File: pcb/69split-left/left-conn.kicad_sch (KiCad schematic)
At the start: 1 part, among them J1 USB_C_Receptacle

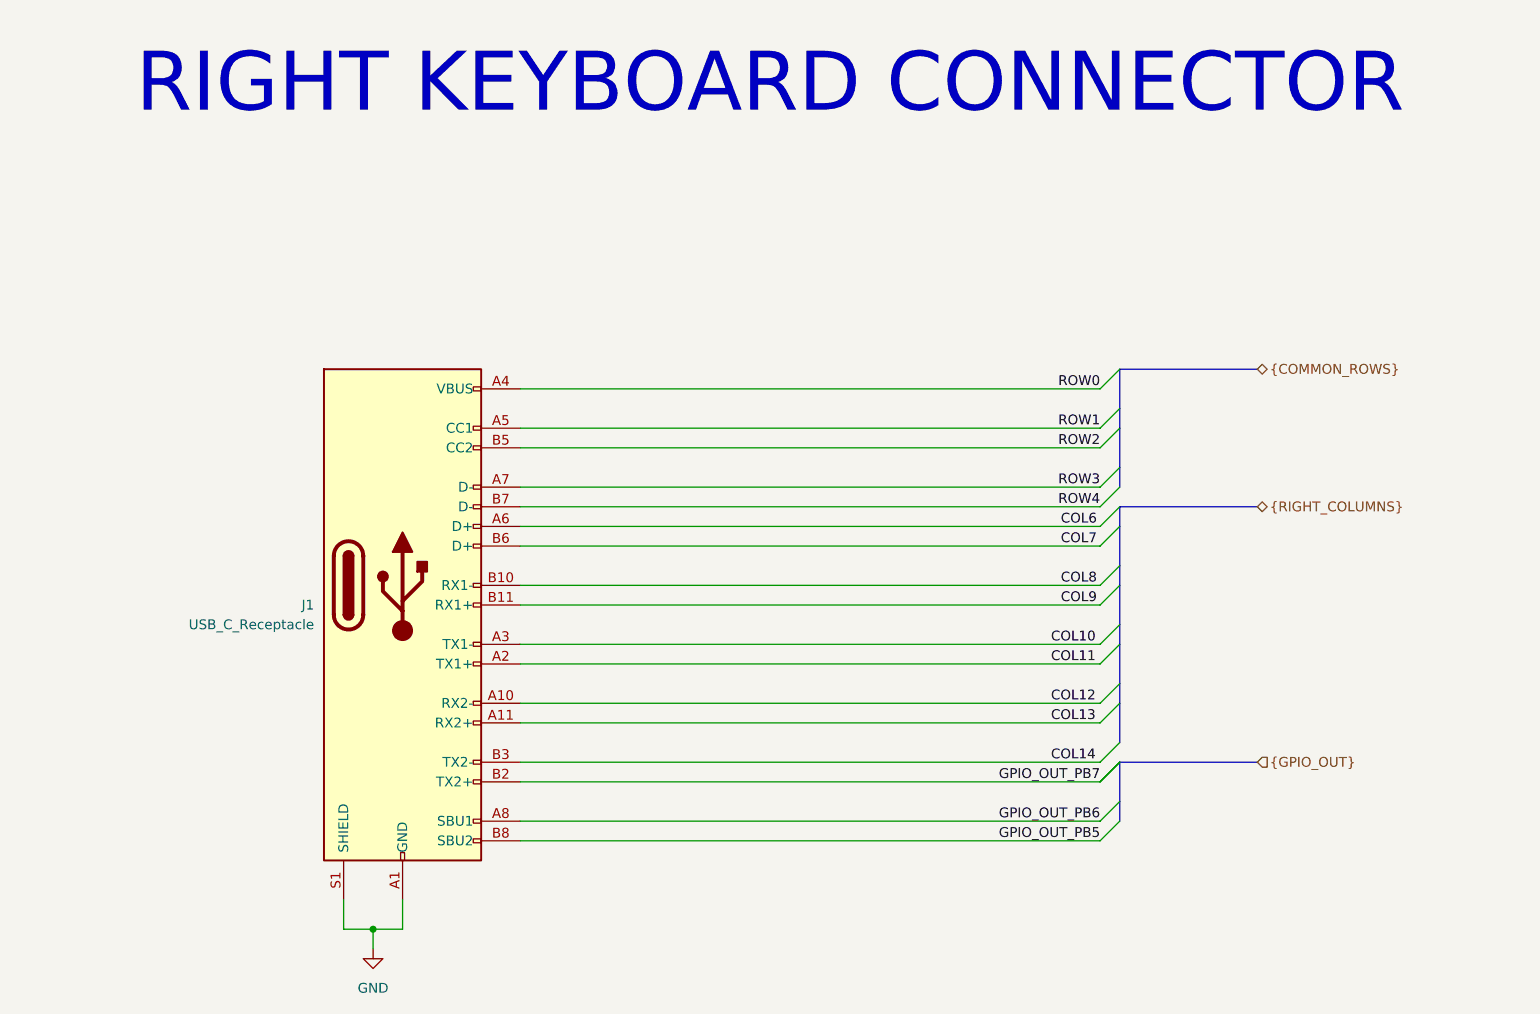
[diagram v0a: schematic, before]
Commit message: Moved things around so it's less confusing.
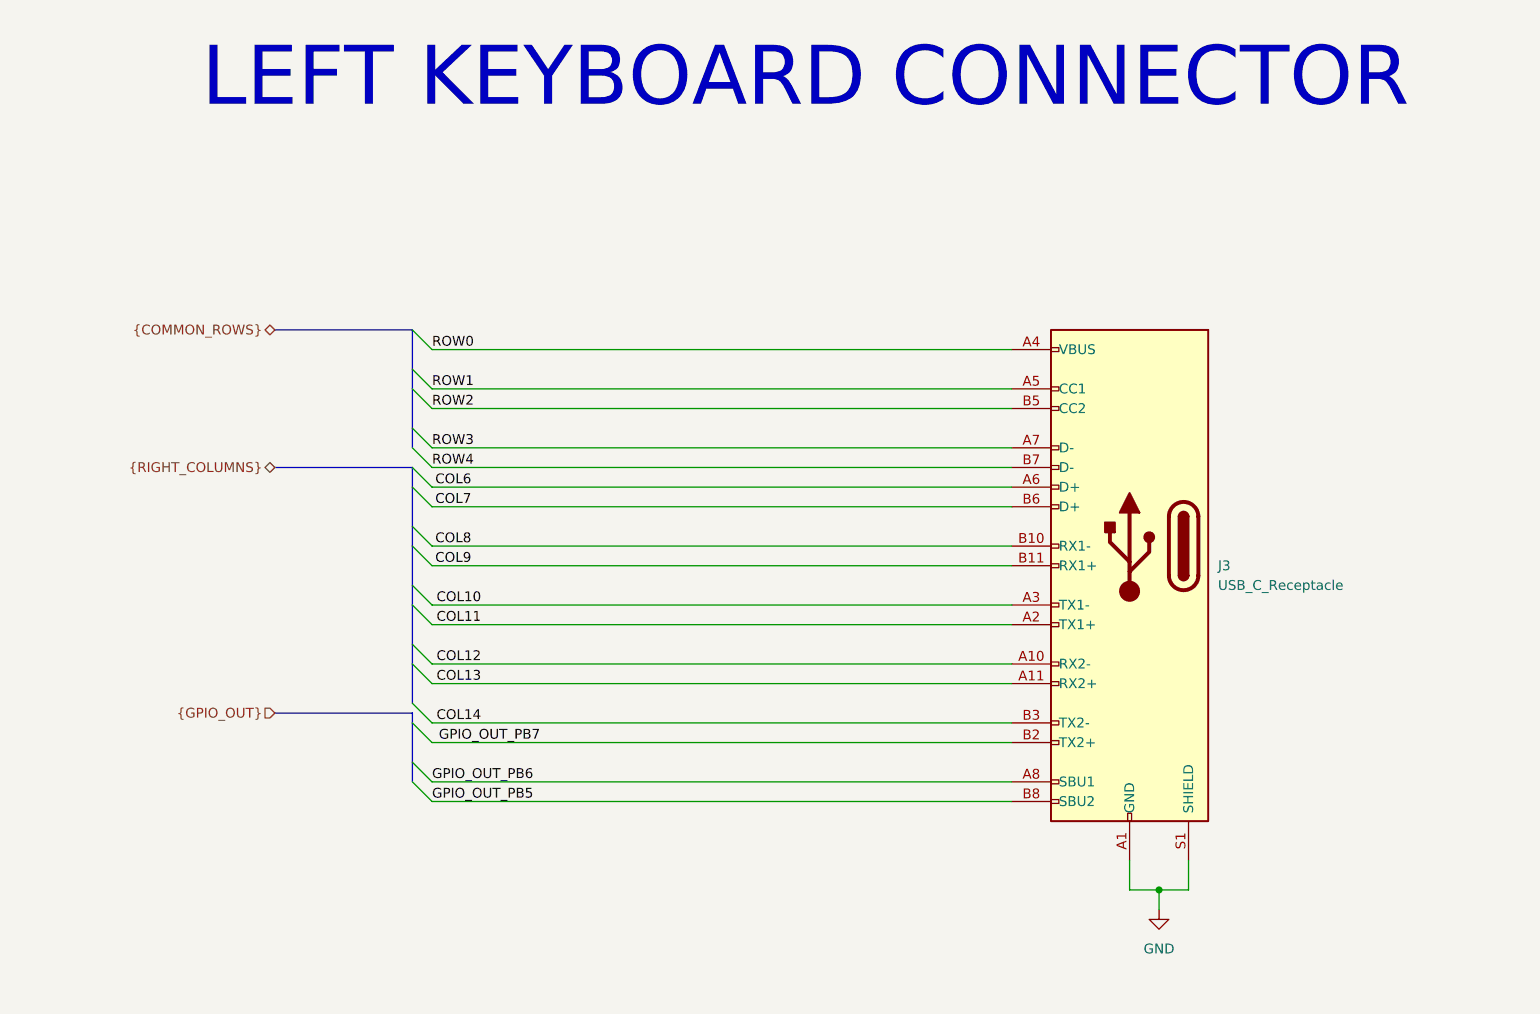
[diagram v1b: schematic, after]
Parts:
- removed J1: USB_C_Receptacle, Connector_USB:USB_C_Receptacle_Amphenol_12401548E4-2A, symbol Connector:USB_C_Receptacle
- added J3: USB_C_Receptacle, Connector_USB:USB_C_Receptacle_Amphenol_12401548E4-2A, symbol Connector:USB_C_Receptacle
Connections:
- net COL10: now also J3.A3 (TX1-)
- net COL11: now also J3.A2 (TX1+)
- net COL12: now also J3.A10 (RX2-)
- net COL13: now also J3.A11 (RX2+)
- net COL14: now also J3.B3 (TX2-)
- net COL6: now also J3.A6 (D+)
- net COL7: now also J3.B6 (D+)
- net COL8: now also J3.B10 (RX1-)
- net COL9: now also J3.B11 (RX1+)
- net GND: now also J3.A1 (GND), J3.A12 (GND), J3.B1 (GND), J3.B12 (GND), J3.S1 (SHIELD)
- net GPIO_OUT_PB5: now also J3.B8 (SBU2)
- net GPIO_OUT_PB6: now also J3.A8 (SBU1)
- net GPIO_OUT_PB7: now also J3.B2 (TX2+)
- net ROW0: now also J3.A4 (VBUS), J3.A9 (VBUS), J3.B4 (VBUS), J3.B9 (VBUS)
- net ROW1: now also J3.A5 (CC1)
- net ROW2: now also J3.B5 (CC2)
- net ROW3: now also J3.A7 (D-)
- net ROW4: now also J3.B7 (D-)
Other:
- note added: "LEFT KEYBOARD CONNECTOR"
- note removed: "RIGHT KEYBOARD CONNECTOR"
